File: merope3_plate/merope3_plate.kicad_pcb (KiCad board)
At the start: 2 copper layers, 171.5 x 119.7 mm, 0 parts

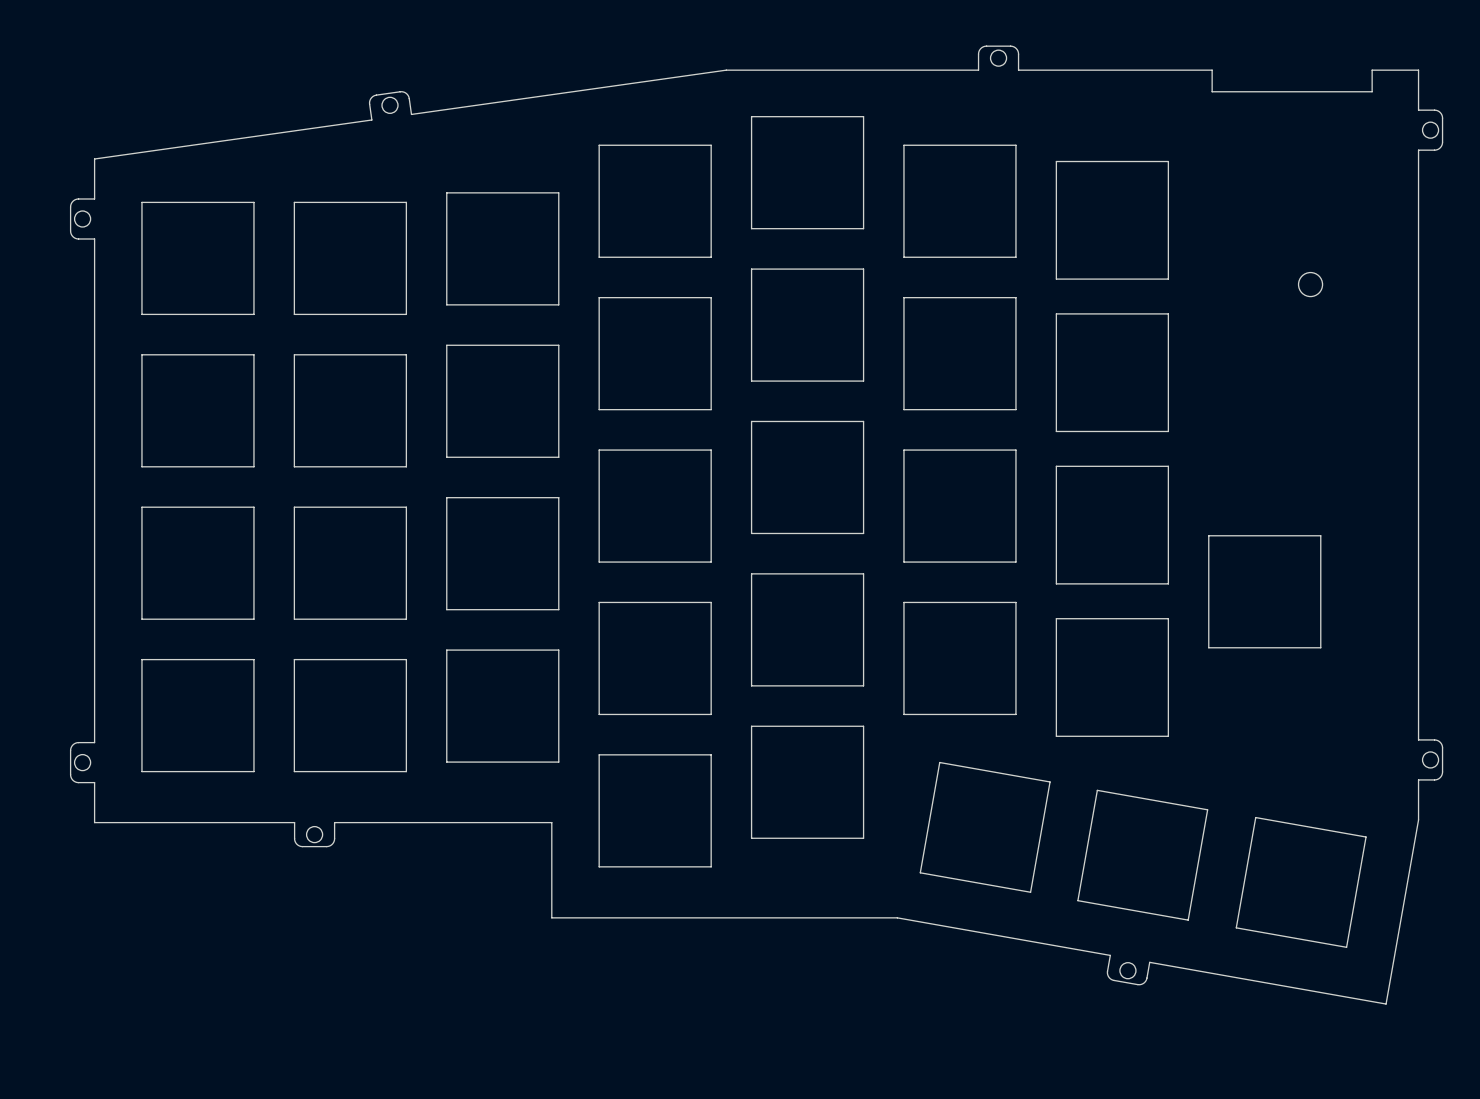
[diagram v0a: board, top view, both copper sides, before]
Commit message: final v1.0
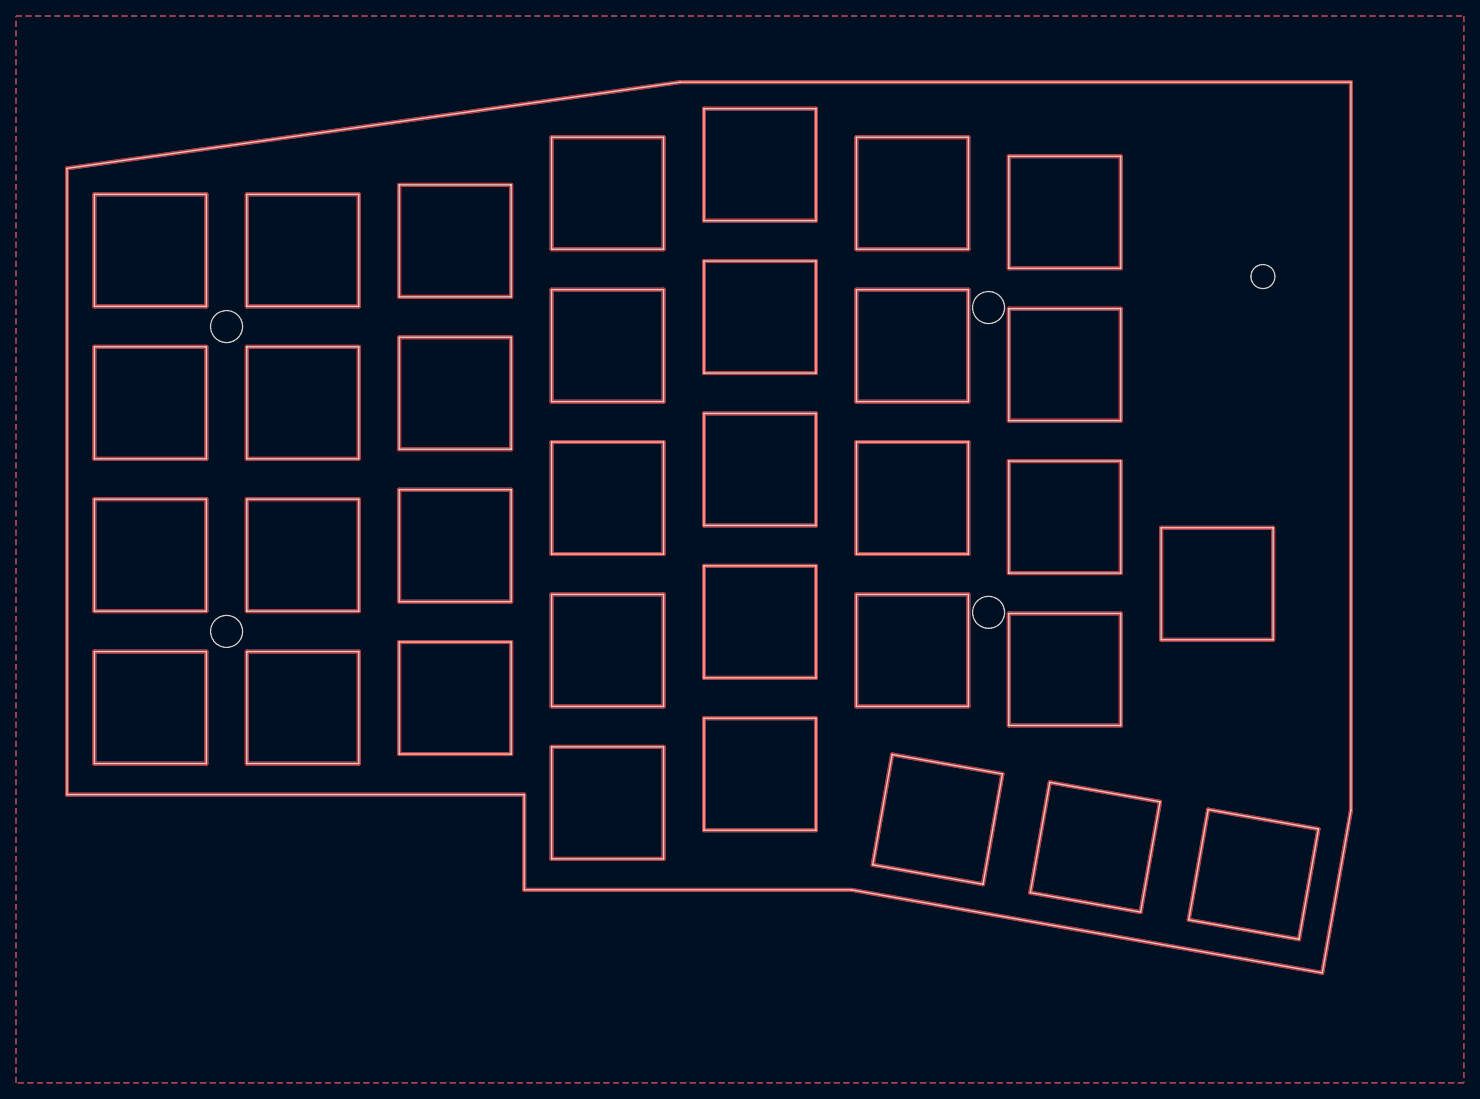
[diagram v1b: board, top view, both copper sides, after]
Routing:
- added copper zone on B.Cu, net (none)
- added copper zone on F.Cu, net (none)
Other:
- board size 171.5 x 119.7 mm -> 160.5 x 111.3 mm
